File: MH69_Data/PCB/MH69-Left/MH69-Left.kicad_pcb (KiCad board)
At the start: 2 copper layers, 163.2 x 92 mm, 85 parts, among them U1 nice_nano

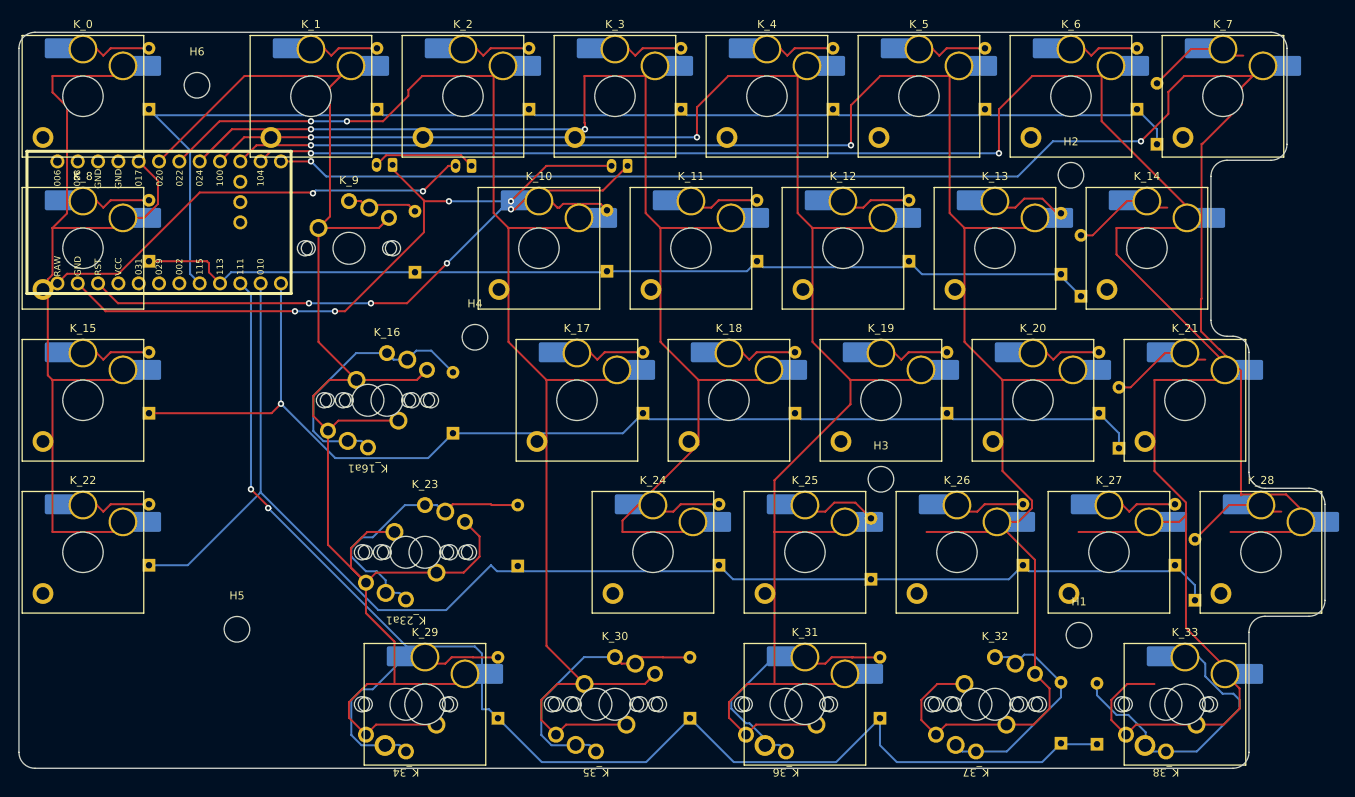
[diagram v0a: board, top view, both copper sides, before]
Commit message: some kicad work
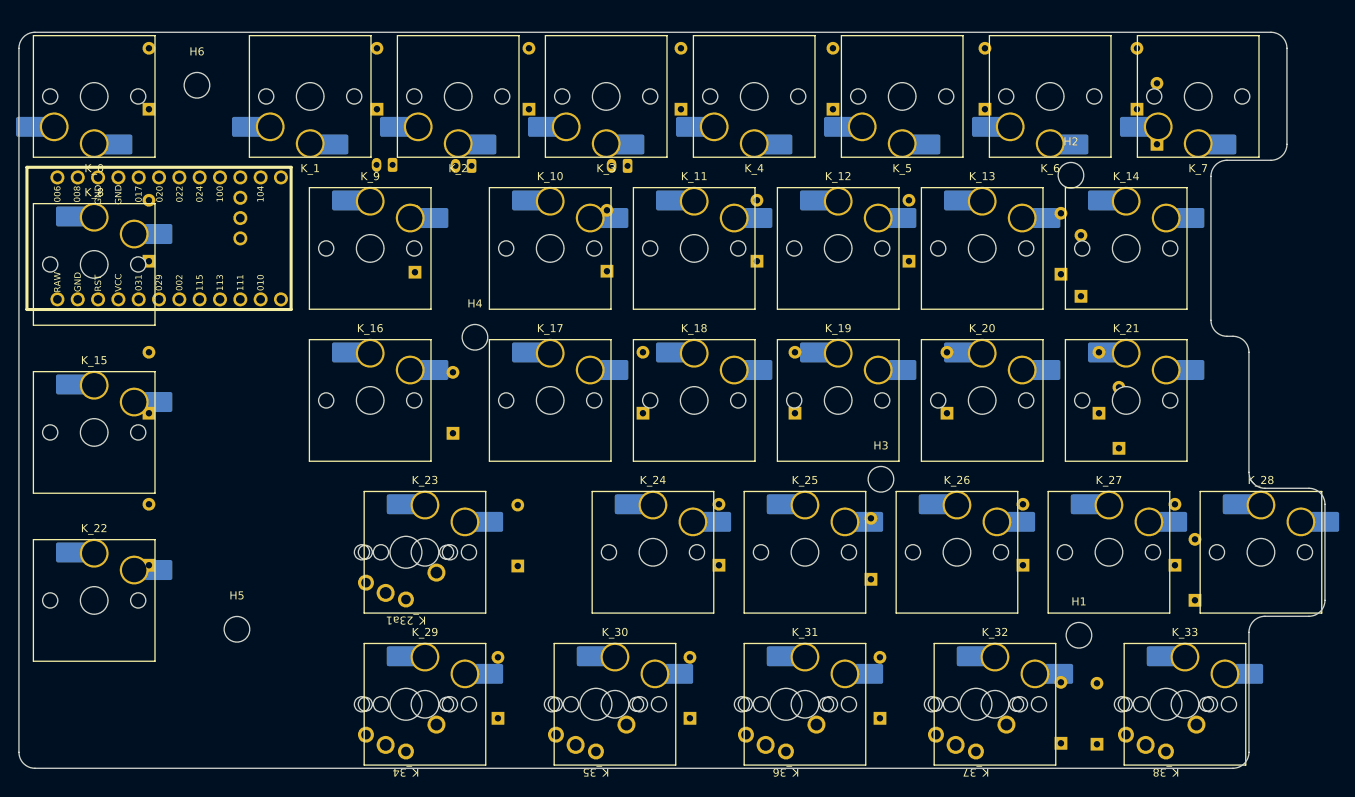
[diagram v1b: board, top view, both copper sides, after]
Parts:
- removed K_16a1: KEYSW, cb:Choc-MX-19mm-1.75u
- K_0, K_1, K_10, K_11, K_12, K_13, K_14, K_15, K_17, K_18, K_19, K_2, K_20, K_21, K_22, K_24, K_25, K_26, K_27, K_28, K_29, K_3, K_31, K_33, K_4, K_5, K_6, K_7, K_8: footprint PCM_Switch_Keyboard_Hotswap_Kailh:SW_Hotswap_Kailh_Choc_V2_Plated_1.00u -> PCM_Switch_Keyboard_Hotswap_Kailh:SW_Hotswap_Kailh_Choc_V1_Plated_1.00u
- K_16, K_23, K_30, K_32, K_9: footprint cb:Choc-MX-19mm-1.5u -> PCM_Switch_Keyboard_Hotswap_Kailh:SW_Hotswap_Kailh_Choc_V1_Plated_1.50u
- moved K_21 7.35 mm to (170.8, 99.8)
- moved K_20 6.35 mm to (152.8, 99.8)
- moved K_22 6.18 mm to (41.8, 124.8)
- moved K_19 5.35 mm to (134.8, 99.8)
- moved K_18 4.35 mm to (116.8, 99.8)
- moved K_15 4.26 mm to (41.8, 103.8)
- moved K_17 3.35 mm to (98.8, 99.8)
- moved K_7 3.10 mm to (179.8, 61.8), turned to 180 degrees
- moved K_9 2.66 mm to (76.3, 80.8)
- moved K_14 2.60 mm to (170.8, 80.8)
- moved K_6 2.60 mm to (161.3, 61.8), turned to 180 degrees
- moved K_8 2.46 mm to (41.8, 82.8)
- moved K_16 2.10 mm to (76.3, 99.8)
- moved K_5 2.10 mm to (142.8, 61.8), turned to 180 degrees
- moved U1 2.00 mm to (51.2, 79.5)
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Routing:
- net col6: track 267.2 -> 0.00 mm, vias 2 -> 0
- net col5: track 243.8 -> 0.00 mm, vias 2 -> 0
- net col4: track 223.2 -> 0.00 mm, vias 2 -> 0
- net col7: track 209.1 -> 0.00 mm, vias 2 -> 0
- net col1: track 208.5 -> 0.00 mm
- net col2: track 176.9 -> 0.00 mm, vias 2 -> 0
- net row3: track 174.7 -> 0.00 mm
- net row4: track 162.8 -> 0.00 mm, vias 2 -> 0
- net col3: track 159.3 -> 0.00 mm, vias 2 -> 0
- net row0: track 157.0 -> 0.00 mm
- net row2: track 146.7 -> 0.00 mm, vias 1 -> 0
- net row1: track 122.0 -> 0.00 mm
- net col0: track 107.7 -> 0.00 mm
- net Net-(Batt1-Pin_1): track 84.1 -> 0.00 mm, vias 4 -> 0
- net Net-(RST1-A): track 74.3 -> 0.00 mm, vias 4 -> 0
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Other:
- board text added: "MH69-L V0"
- board text removed: "CB70S-L v3"
